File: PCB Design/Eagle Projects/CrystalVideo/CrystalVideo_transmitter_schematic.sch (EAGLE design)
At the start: 1 part

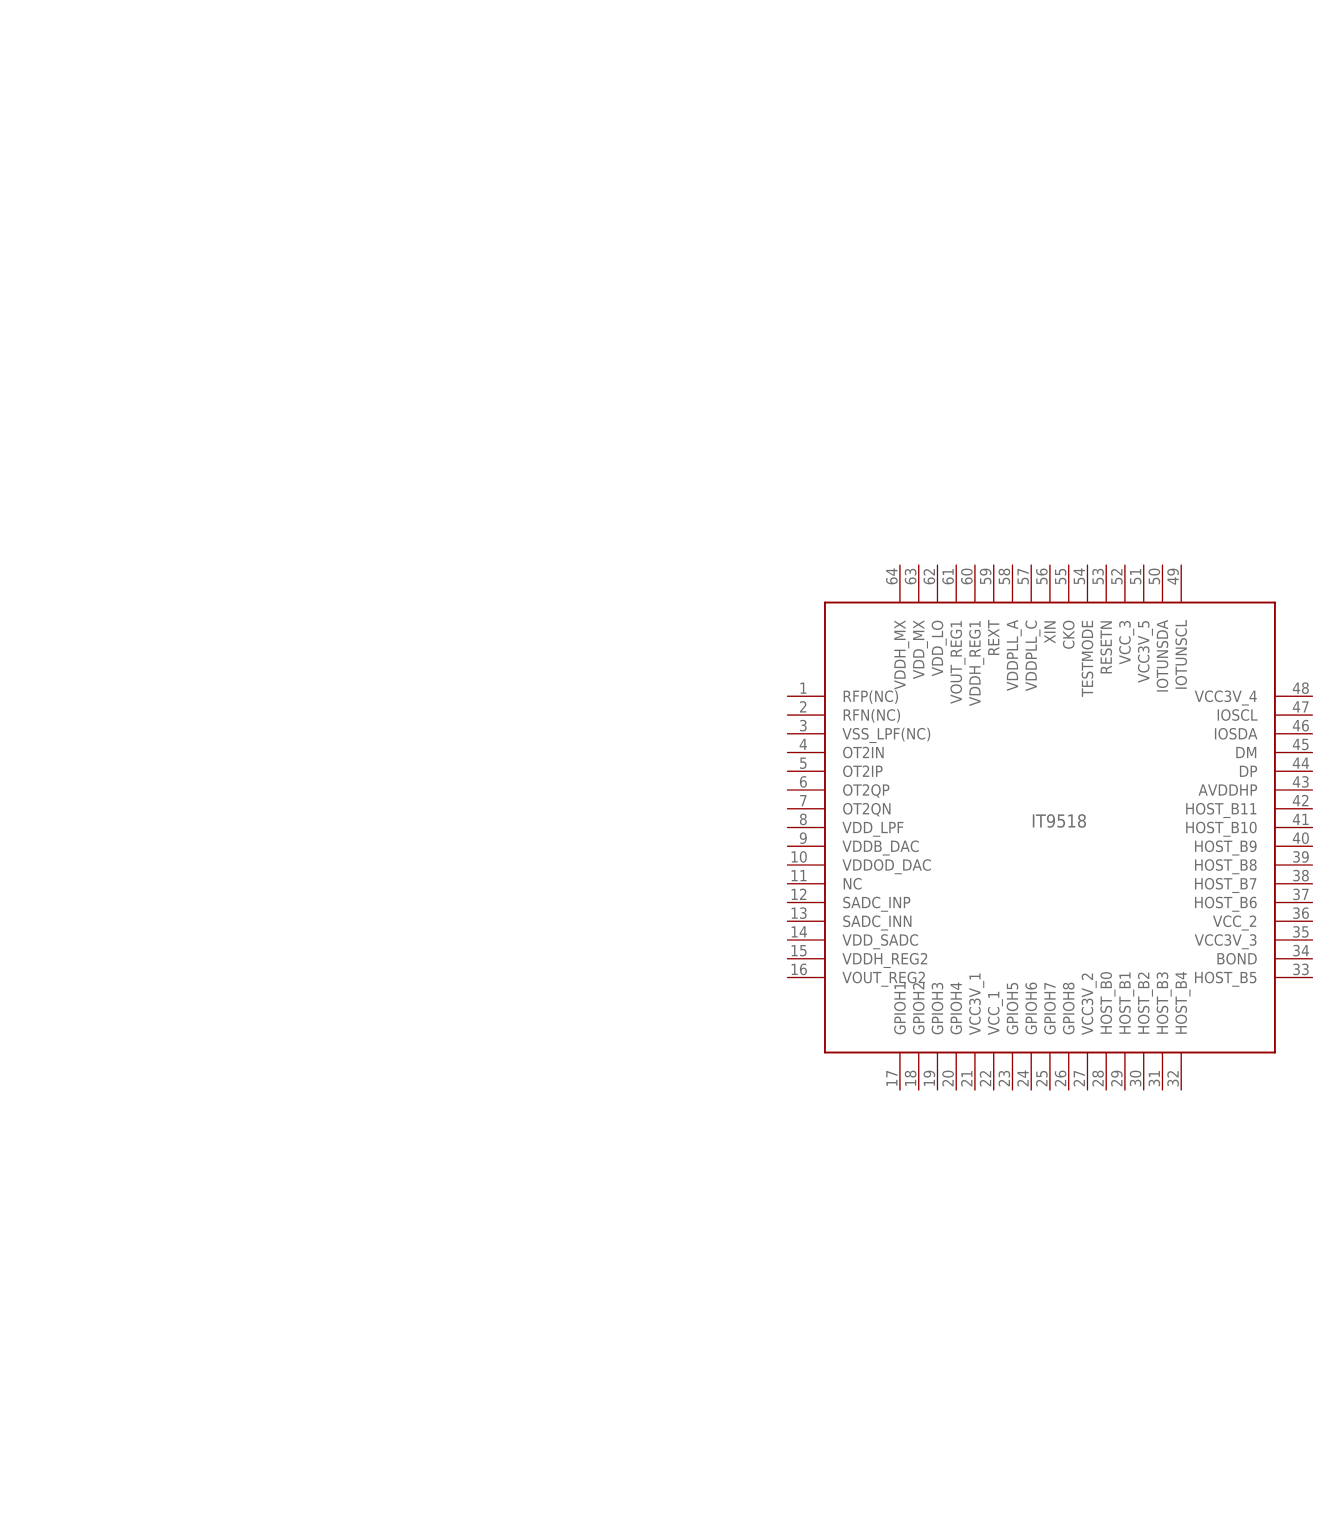
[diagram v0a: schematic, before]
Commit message: PCB schematics
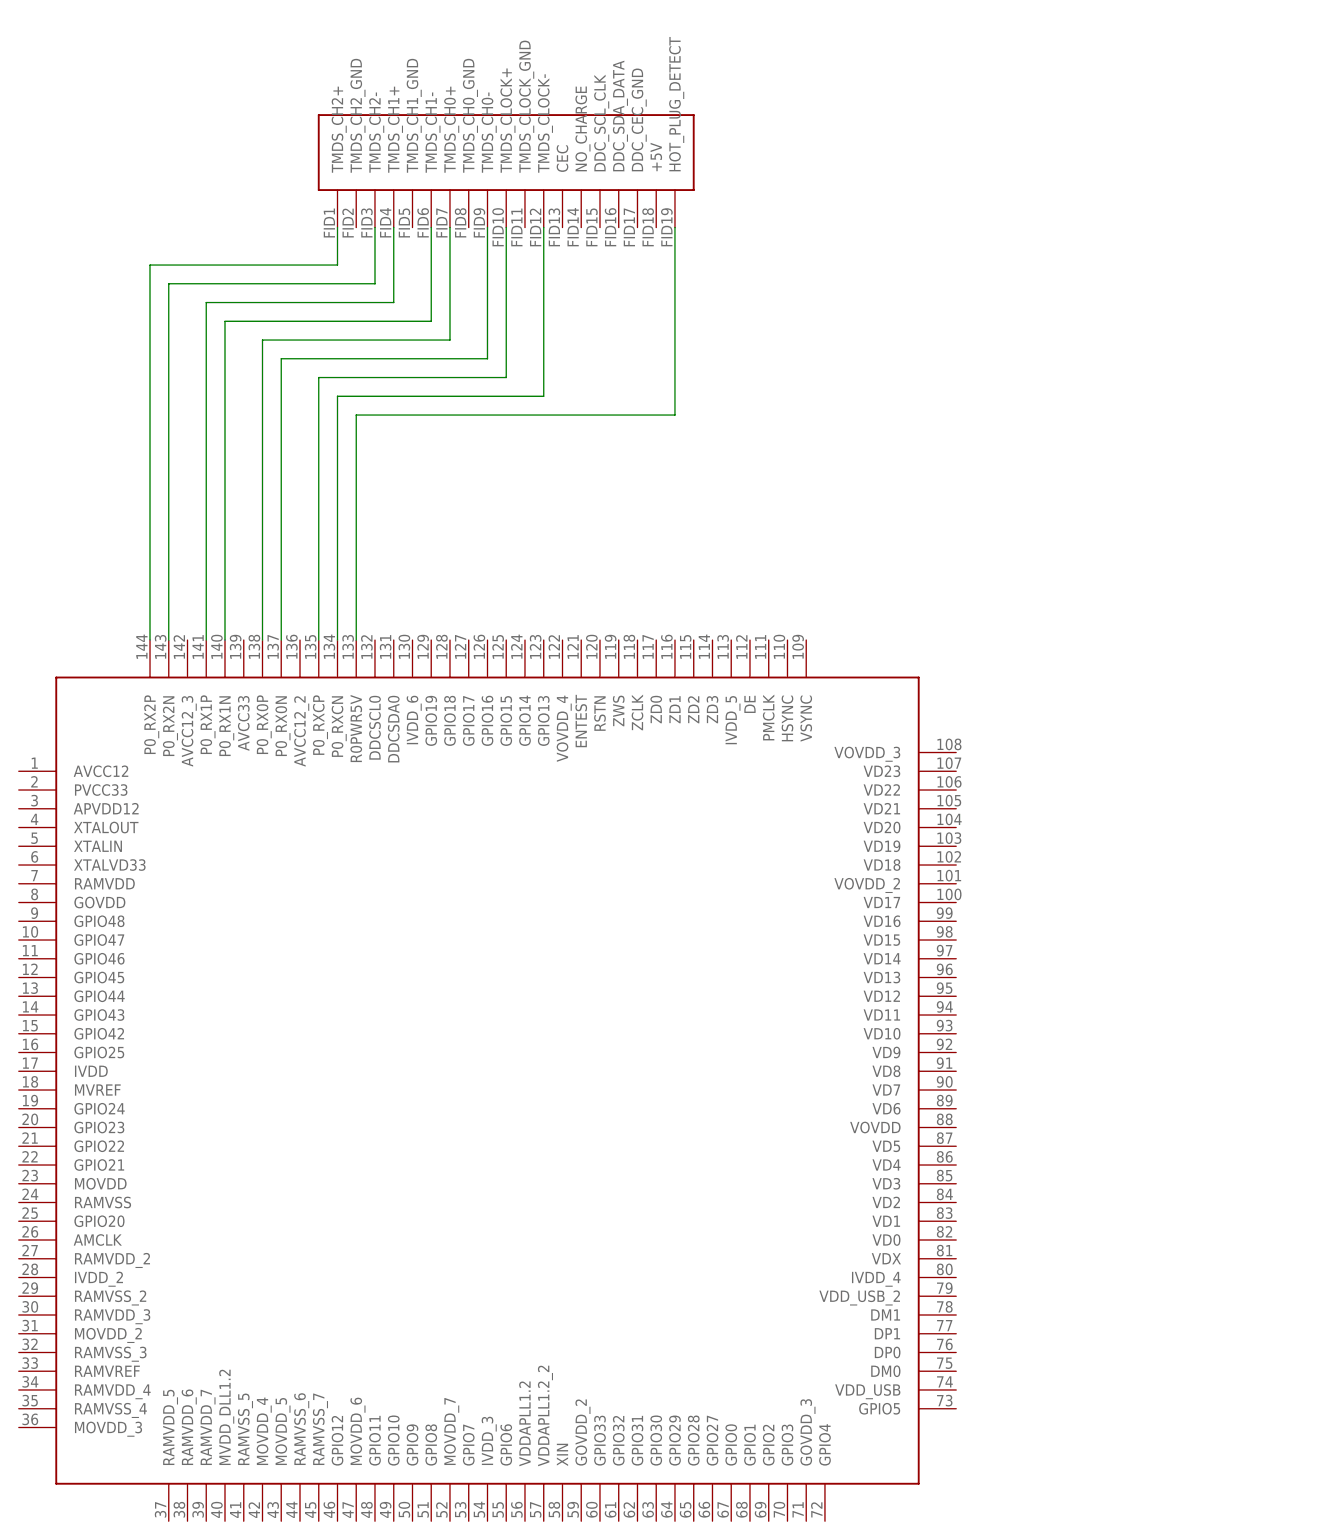
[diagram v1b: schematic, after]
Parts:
- added U$2: IT9919, CrystalVideo:IT9919
- U$1: value IT9518 -> HDMI_MOLEX; device CrystalVideo:IT9518 -> CrystalVideo:HDMI_MOLEX
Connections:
- new net N$1: U$1.TMDS_CH0-, U$2.P0_RX0N
- new net N$2: U$1.TMDS_CH0+, U$2.P0_RX0P
- new net N$3: U$1.TMDS_CH1-, U$2.P0_RX1N
- new net N$4: U$1.TMDS_CH1+, U$2.P0_RX1P
- new net N$5: U$1.TMDS_CH2-, U$2.P0_RX2N
- new net N$6: U$1.TMDS_CH2+, U$2.P0_RX2P
- new net N$7: U$1.TMDS_CLOCK-, U$2.P0_RXCN
- new net N$8: U$1.TMDS_CLOCK+, U$2.P0_RXCP
- new net N$9: U$1.HOT_PLUG_DETECT, U$2.R0PWR5V
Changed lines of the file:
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@@
 </classes>
 <parts>
-<part name="U$1" library="CrystalVideo" deviceset="IT9518" device=""/>
+<part name="U$1" library="CrystalVideo" deviceset="HDMI_MOLEX" device=""/>
+<part name="U$2" library="CrystalVideo" deviceset="IT9919" device=""/>
 </parts>
 <sheets>
@@
 </plain>
 <instances>
-<instance part="U$1" gate="G$1" x="73.66" y="43.18"/>
+<instance part="U$1" gate="G$1" x="12.7" y="139.7" rot="MR180"/>
+<instance part="U$2" gate="G$1" x="2.54" y="10.16"/>
 </instances>
 <busses>
 </busses>
 <nets>
+<net name="N$1" class="0">
+<segment>
+<pinref part="U$1" gate="G$1" pin="TMDS_CH0-"/>
+<wire x1="-2.54" y1="124.46" x2="-2.54" y2="106.68" width="0.1524" layer="91"/>
+<pinref part="U$2" gate="G$1" pin="P0_RX0N"/>
+<wire x1="-2.54" y1="106.68" x2="-30.48" y2="106.68" width="0.1524" layer="91"/>
+<wire x1="-30.48" y1="106.68" x2="-30.48" y2="68.58" width="0.1524" layer="91"/>
+</segment>
+</net>
+<net name="N$2" class="0">
+<segment>
+<pinref part="U$1" gate="G$1" pin="TMDS_CH0+"/>
+<wire x1="-7.62" y1="124.46" x2="-7.62" y2="109.22" width="0.1524" layer="91"/>
+<wire x1="-7.62" y1="109.22" x2="-33.02" y2="109.22" width="0.1524" layer="91"/>
+<pinref part="U$2" gate="G$1" pin="P0_RX0P"/>
+<wire x1="-33.02" y1="109.22" x2="-33.02" y2="68.58" width="0.1524" layer="91"/>
+</segment>
+</net>
+<net name="N$3" class="0">
+<segment>
+<pinref part="U$1" gate="G$1" pin="TMDS_CH1-"/>
+<wire x1="-10.16" y1="124.46" x2="-10.16" y2="111.76" width="0.1524" layer="91"/>
+<wire x1="-10.16" y1="111.76" x2="-38.1" y2="111.76" width="0.1524" layer="91"/>
+<pinref part="U$2" gate="G$1" pin="P0_RX1N"/>
+<wire x1="-38.1" y1="111.76" x2="-38.1" y2="68.58" width="0.1524" layer="91"/>
+</segment>
+</net>
+<net name="N$4" class="0">
+<segment>
+<pinref part="U$1" gate="G$1" pin="TMDS_CH1+"/>
+<wire x1="-15.24" y1="124.46" x2="-15.24" y2="114.3" width="0.1524" layer="91"/>
+<pinref part="U$2" gate="G$1" pin="P0_RX1P"/>
+<wire x1="-15.24" y1="114.3" x2="-40.64" y2="114.3" width="0.1524" layer="91"/>
+<wire x1="-40.64" y1="114.3" x2="-40.64" y2="68.58" width="0.1524" layer="91"/>
+</segment>
+</net>
+<net name="N$5" class="0">
+<segment>
+<pinref part="U$1" gate="G$1" pin="TMDS_CH2-"/>
+<wire x1="-17.78" y1="124.46" x2="-17.78" y2="116.84" width="0.1524" layer="91"/>
+<pinref part="U$2" gate="G$1" pin="P0_RX2N"/>
+<wire x1="-17.78" y1="116.84" x2="-45.72" y2="116.84" width="0.1524" layer="91"/>
+<wire x1="-45.72" y1="116.84" x2="-45.72" y2="68.58" width="0.1524" layer="91"/>
+</segment>
+</net>
+<net name="N$6" class="0">
+<segment>
+<pinref part="U$1" gate="G$1" pin="TMDS_CH2+"/>
+<wire x1="-22.86" y1="124.46" x2="-22.86" y2="119.38" width="0.1524" layer="91"/>
+<pinref part="U$2" gate="G$1" pin="P0_RX2P"/>
+<wire x1="-22.86" y1="119.38" x2="-48.26" y2="119.38" width="0.1524" layer="91"/>
+<wire x1="-48.26" y1="119.38" x2="-48.26" y2="68.58" width="0.1524" layer="91"/>
+</segment>
+</net>
+<net name="N$7" class="0">
+<segment>
+<pinref part="U$1" gate="G$1" pin="TMDS_CLOCK-"/>
+<wire x1="5.08" y1="124.46" x2="5.08" y2="101.6" width="0.1524" layer="91"/>
+<pinref part="U$2" gate="G$1" pin="P0_RXCN"/>
+<wire x1="5.08" y1="101.6" x2="-22.86" y2="101.6" width="0.1524" layer="91"/>
+<wire x1="-22.86" y1="101.6" x2="-22.86" y2="68.58" width="0.1524" layer="91"/>
+</segment>
+</net>
+<net name="N$8" class="0">
+<segment>
+<pinref part="U$1" gate="G$1" pin="TMDS_CLOCK+"/>
+<wire x1="0" y1="124.46" x2="0" y2="104.14" width="0.1524" layer="91"/>
+<pinref part="U$2" gate="G$1" pin="P0_RXCP"/>
+<wire x1="0" y1="104.14" x2="-25.4" y2="104.14" width="0.1524" layer="91"/>
+<wire x1="-25.4" y1="104.14" x2="-25.4" y2="68.58" width="0.1524" layer="91"/>
+</segment>
+</net>
+<net name="N$9" class="0">
+<segment>
+<pinref part="U$1" gate="G$1" pin="HOT_PLUG_DETECT"/>
+<wire x1="22.86" y1="124.46" x2="22.86" y2="99.06" width="0.1524" layer="91"/>
+<pinref part="U$2" gate="G$1" pin="R0PWR5V"/>
+<wire x1="22.86" y1="99.06" x2="-20.32" y2="99.06" width="0.1524" layer="91"/>
+<wire x1="-20.32" y1="99.06" x2="-20.32" y2="68.58" width="0.1524" layer="91"/>
+</segment>
+</net>
 </nets>
 </sheet>
